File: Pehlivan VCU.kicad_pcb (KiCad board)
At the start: 2 copper layers, 85.7 x 86.6 mm, 58 parts, among them J1 PWR_IN, J2 DEBUG, J3 SD_CARD MODULE, J4 Headlights, J5 Nextion, J6 LORA, J7 Blinker, J8 CAN, J9 Stop, U1 L7805, U2 STM32G431C8Tx, U3 LM1117MP-3.3, U4 BTS432, U5 BTS432, U6 BTS432, U7 BTS432, U8 TJA1051T-3, U9 BTS432, Y1 16MHz 18pF

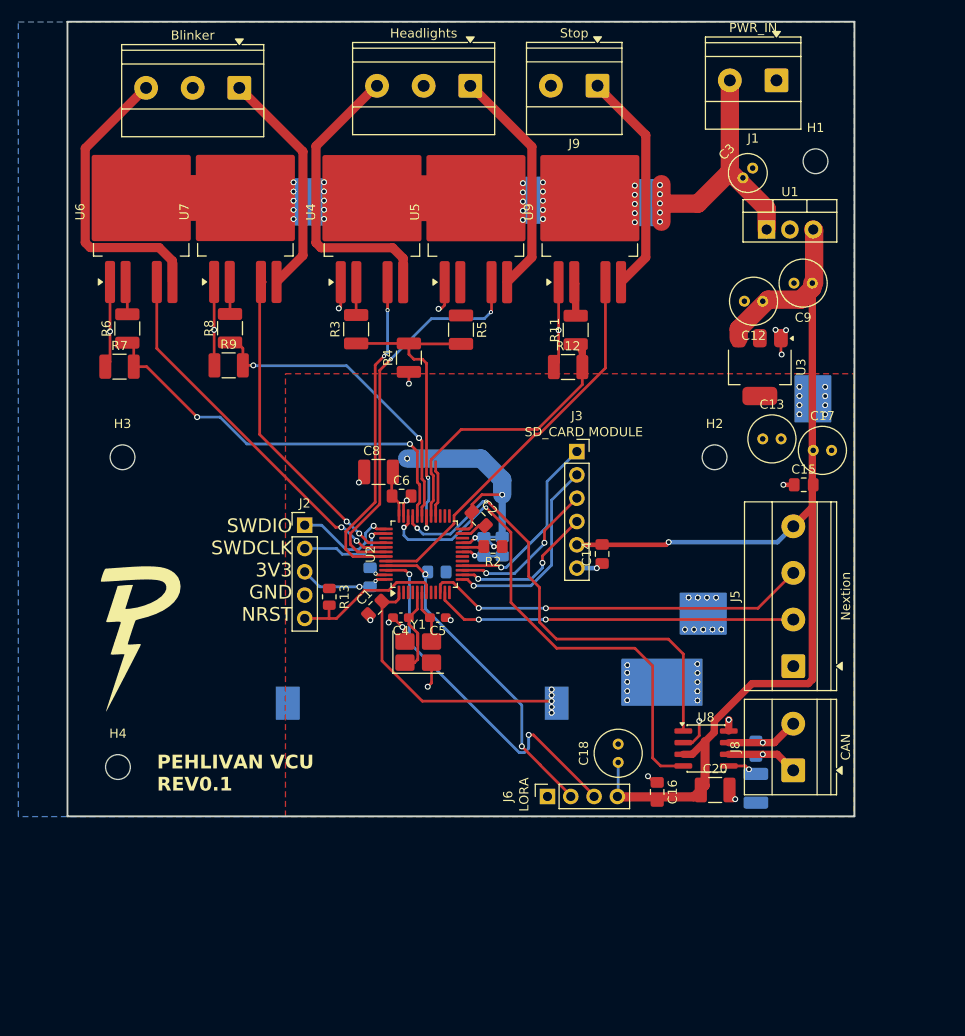
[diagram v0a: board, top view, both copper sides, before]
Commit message: changes
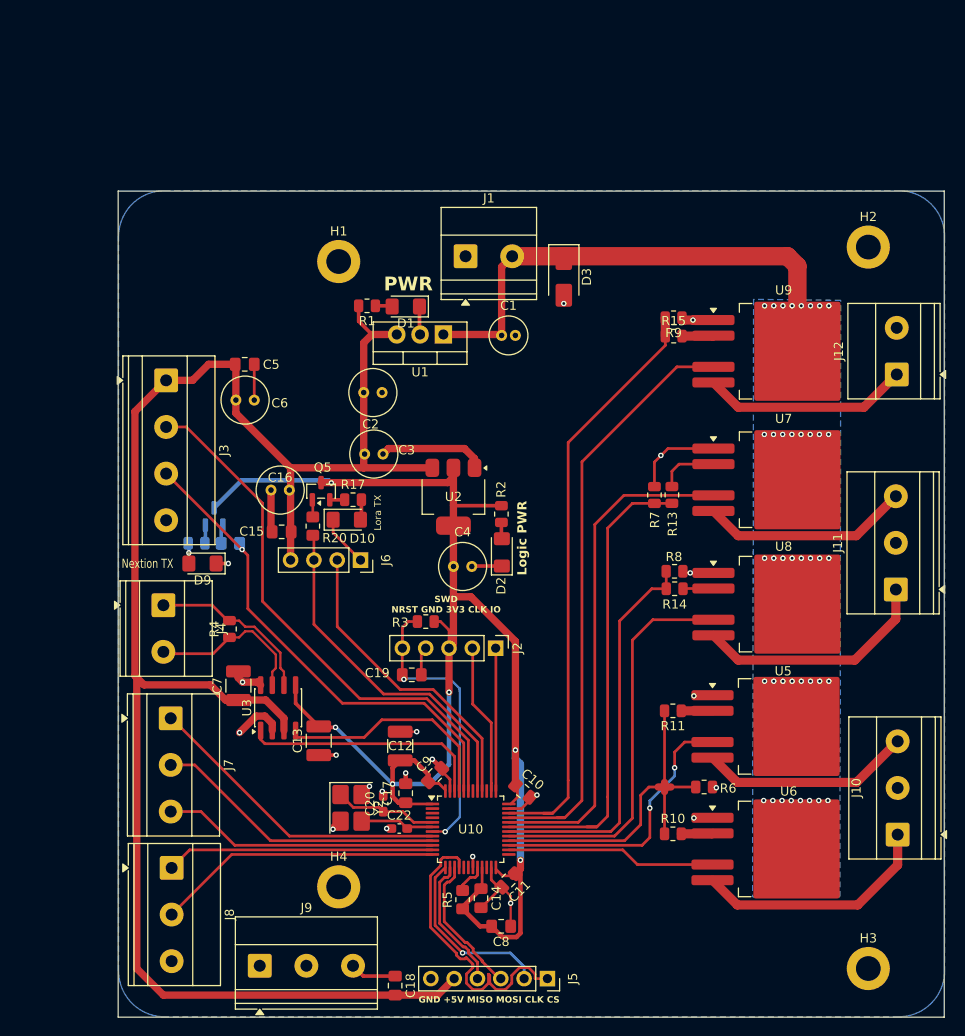
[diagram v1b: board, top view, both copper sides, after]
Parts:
- removed BT1: Battery_Cell, Battery:BatteryHolder_Keystone_1060_1x2032
- removed G***: LOGO, LOGO
- removed R12: 10k, Resistor_SMD:R_1210_3225Metric_Pad1.30x2.65mm_HandSolder
- removed U4: BTS432, Package_TO_SOT_SMD:TO-263-4
- removed Y1: 16MHz 18pF, Crystal:Crystal_SMD_3225-4Pin_3.2x2.5mm_HandSoldering
- added C22: 26pF, Capacitor_SMD:C_0603_1608Metric_Pad1.08x0.95mm_HandSolder, F.Cu at (133.9, 129.4)
- added D1: LED, LED_SMD:LED_1206_3216Metric_Pad1.42x1.75mm_HandSolder, F.Cu at (134.6, 72.6)
- added D10: LED, LED_SMD:LED_1206_3216Metric_Pad1.42x1.75mm_HandSolder, F.Cu at (128.2, 95.8)
- added D2: LED, LED_SMD:LED_1206_3216Metric_Pad1.42x1.75mm_HandSolder, F.Cu at (145.1, 99.4)
- added D3: SMAJ16CA, Diode_SMD:D_SMA, F.Cu at (151.8, 69.3)
- added D9: LED, LED_SMD:LED_1206_3216Metric_Pad1.42x1.75mm_HandSolder, F.Cu at (112.5, 100.6)
- added J10: Headlights, TerminalBlock_Phoenix:TerminalBlock_Phoenix_MKDS-1,5-3-5.08_1x03_P5.08mm_Horizontal, F.Cu at (188.2, 130.1)
- added J11: Blinker, TerminalBlock_Phoenix:TerminalBlock_Phoenix_MKDS-1,5-3-5.08_1x03_P5.08mm_Horizontal, F.Cu at (188.0, 103.4)
- added J12: Stop, TerminalBlock_Phoenix:TerminalBlock_Phoenix_MKDS-1,5-2-5.08_1x02_P5.08mm_Horizontal, F.Cu at (188.1, 80.0)
- added Q4: BC817, Package_TO_SOT_SMD:SOT-23, B.Cu at (113.7, 95.5)
- added Q5: BC817, Package_TO_SOT_SMD:SOT-23, F.Cu at (125.4, 92.7)
- added R14: 4k7, Resistor_SMD:R_0805_2012Metric, F.Cu at (163.9, 103.3)
- added R15: 4k7, Resistor_SMD:R_0805_2012Metric, F.Cu at (163.8, 75.8)
- added R16: 1k, Resistor_SMD:R_0805_2012Metric, B.Cu at (111.8, 98.4)
- added R17: 1k, Resistor_SMD:R_0805_2012Metric, F.Cu at (128.9, 93.6)
- added R19: 4.7K, Resistor_SMD:R_0805_2012Metric_Pad1.20x1.40mm_HandSolder, B.Cu at (115.5, 98.4)
- added R20: 4.7K, Resistor_SMD:R_0805_2012Metric_Pad1.20x1.40mm_HandSolder, F.Cu at (124.5, 96.5)
- added U10: STM32G431C8Tx, Package_QFP:LQFP-48_7x7mm_P0.5mm, F.Cu at (141.7, 129.5)
- added Y2: 16MHz 18pF, Crystal:Crystal_SMD_3225-4Pin_3.2x2.5mm_HandSoldering, F.Cu at (128.7, 127.2)
- C1: value 100nF -> 100uF; footprint Capacitor_SMD:C_0805_2012Metric_Pad1.18x1.45mm_HandSolder -> Capacitor_THT:C_Radial_D4.0mm_H7.0mm_P1.50mm
- C10: moved to F.Cu
- C11: value 10uF -> 100nF; moved to F.Cu
- C12: footprint Capacitor_THT:C_Radial_D5.0mm_H5.0mm_P2.00mm -> Capacitor_SMD:C_1210_3225Metric_Pad1.33x2.70mm_HandSolder
- C13: value 1uF -> 100nF; footprint Capacitor_THT:C_Radial_D5.0mm_H5.0mm_P2.00mm -> Capacitor_SMD:C_1210_3225Metric_Pad1.33x2.70mm_HandSolder
- C16, C2, C6: value 100nF -> 10uF; footprint Capacitor_SMD:C_0805_2012Metric_Pad1.18x1.45mm_HandSolder -> Capacitor_THT:C_Radial_D5.0mm_H5.0mm_P2.00mm
- C17, C18, C9: value 10uF -> 100nF; footprint Capacitor_THT:C_Radial_D5.0mm_H5.0mm_P2.00mm -> Capacitor_SMD:C_0805_2012Metric_Pad1.18x1.45mm_HandSolder
- C19: footprint Capacitor_SMD:C_1210_3225Metric_Pad1.33x2.70mm_HandSolder -> Capacitor_SMD:C_0805_2012Metric_Pad1.18x1.45mm_HandSolder; moved to F.Cu
- C20: value 100nF -> 26pF; footprint Capacitor_SMD:C_1210_3225Metric_Pad1.33x2.70mm_HandSolder -> Capacitor_SMD:C_0603_1608Metric_Pad1.08x0.95mm_HandSolder
- C3: value 100uF -> 10uF; footprint Capacitor_THT:C_Radial_D4.0mm_H7.0mm_P1.50mm -> Capacitor_THT:C_Radial_D5.0mm_H5.0mm_P2.00mm
- C4: value 26pF -> 1uF; footprint Capacitor_SMD:C_0603_1608Metric_Pad1.08x0.95mm_HandSolder -> Capacitor_THT:C_Radial_D5.0mm_H5.0mm_P2.00mm
- C5: value 26pF -> 100nF; footprint Capacitor_SMD:C_0603_1608Metric_Pad1.08x0.95mm_HandSolder -> Capacitor_SMD:C_0805_2012Metric_Pad1.18x1.45mm_HandSolder
- C7: footprint Capacitor_SMD:C_0805_2012Metric_Pad1.18x1.45mm_HandSolder -> Capacitor_SMD:C_1210_3225Metric_Pad1.33x2.70mm_HandSolder; moved to F.Cu
- C8: footprint Capacitor_SMD:C_1210_3225Metric_Pad1.33x2.70mm_HandSolder -> Capacitor_SMD:C_0805_2012Metric_Pad1.18x1.45mm_HandSolder
- H1, H2, H3, H4: footprint MountingHole:MountingHole_2.7mm_M2.5 -> MountingHole:MountingHole_2.7mm_M2.5_DIN965_Pad
- J3: value SD_CARD MODULE -> Nextion; footprint Connector_PinSocket_2.54mm:PinSocket_1x06_P2.54mm_Vertical -> TerminalBlock_Phoenix:TerminalBlock_Phoenix_MKDS-1,5-4-5.08_1x04_P5.08mm_Horizontal
- J4: value Headlights -> CAN; footprint TerminalBlock_Phoenix:TerminalBlock_Phoenix_MKDS-1,5-3-5.08_1x03_P5.08mm_Horizontal -> TerminalBlock_Phoenix:TerminalBlock_Phoenix_MKDS-1,5-2-5.08_1x02_P5.08mm_Horizontal
- J5: value Nextion -> SD_CARD MODULE; footprint TerminalBlock_Phoenix:TerminalBlock_Phoenix_MKDS-1,5-4-5.08_1x04_P5.08mm_Horizontal -> Connector_PinSocket_2.54mm:PinSocket_1x06_P2.54mm_Vertical
- J7: value Blinker -> IN1
- J8: value CAN -> IN2; footprint TerminalBlock_Phoenix:TerminalBlock_Phoenix_MKDS-1,5-2-5.08_1x02_P5.08mm_Horizontal -> TerminalBlock_Phoenix:TerminalBlock_Phoenix_MKDS-1,5-3-5.08_1x03_P5.08mm_Horizontal
- J9: value Stop -> GND; footprint TerminalBlock_Phoenix:TerminalBlock_Phoenix_MKDS-1,5-2-5.08_1x02_P5.08mm_Horizontal -> TerminalBlock_Phoenix:TerminalBlock_Phoenix_MKDS-1,5-3-5.08_1x03_P5.08mm_Horizontal
- R1: value 10k -> 1k; footprint Resistor_SMD:R_0805_2012Metric_Pad1.20x1.40mm_HandSolder -> Resistor_SMD:R_0805_2012Metric; moved to F.Cu
- R10: value 100R -> 4k7; moved to F.Cu
- R11, R7, R9: footprint Resistor_SMD:R_1210_3225Metric_Pad1.30x2.65mm_HandSolder -> Resistor_SMD:R_0805_2012Metric
- R13: value 10k -> 4k7
- R2: value 47R -> 1k; footprint Resistor_SMD:R_0805_2012Metric_Pad1.20x1.40mm_HandSolder -> Resistor_SMD:R_0805_2012Metric
- R3, R6, R8: value 4k7 -> 10k; footprint Resistor_SMD:R_1210_3225Metric_Pad1.30x2.65mm_HandSolder -> Resistor_SMD:R_0805_2012Metric
- R4: value 10k -> 100R; footprint Resistor_SMD:R_1210_3225Metric_Pad1.30x2.65mm_HandSolder -> Resistor_SMD:R_0805_2012Metric
- R5: value 4k7 -> 47R; footprint Resistor_SMD:R_1210_3225Metric_Pad1.30x2.65mm_HandSolder -> Resistor_SMD:R_0805_2012Metric_Pad1.20x1.40mm_HandSolder
- U2: value STM32G431C8Tx -> LM1117MP-3.3; footprint Package_QFP:LQFP-48_7x7mm_P0.5mm -> Package_TO_SOT_SMD:SOT-223-3_TabPin2
- U3: value LM1117MP-3.3 -> TJA1051T-3; footprint Package_TO_SOT_SMD:SOT-223-3_TabPin2 -> Package_SO:SOIC-8_3.9x4.9mm_P1.27mm
- U8: value TJA1051T-3 -> BTS432; footprint Package_SO:SOIC-8_3.9x4.9mm_P1.27mm -> Package_TO_SOT_SMD:TO-263-4
- moved J9 102.7 mm to (118.7, 144.4), turned to 0 degrees
- moved H3 98.5 mm to (185.0, 144.7)
- moved U6 98.5 mm to (175.7, 131.7), turned to 0 degrees
- moved R6 80.3 mm to (167.1, 124.9), turned to 180 degrees
- moved J7 69.1 mm to (109.0, 117.4), turned to -90 degrees
- moved J8 68.5 mm to (109.1, 133.7), turned to -90 degrees
- moved C9 67.5 mm to (137.8, 123.6), turned to 45 degrees
- moved J4 65.7 mm to (108.2, 105.1), turned to -90 degrees
- moved U7 65.5 mm to (175.8, 91.5), turned to 0 degrees
- moved U5 65.3 mm to (175.7, 118.3), turned to 0 degrees
- moved U3 64.3 mm to (120.7, 116.3), turned to 90 degrees
- moved C12 62.5 mm to (134.0, 120.5), turned to -90 degrees
- moved R5 62.1 mm to (140.8, 137.2), turned to 90 degrees
- moved R7 59.9 mm to (161.7, 93.1), turned to -90 degrees
- moved C13 58.5 mm to (125.1, 119.9), turned to 90 degrees
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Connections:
- C1 pad 1: GND -> VCC
- C1 pad 2: /VBAT -> GND
- C11 pad 1: GND -> +3V3
- C11 pad 2: +3V3 -> GND
- C12 pad 1: +5V -> GND
- C12 pad 2: GND -> +3V3
- C13 pad 1: +3V3 -> GND
- C13 pad 2: GND -> +3V3
- C14 pad 1: GND -> +3V3
- C14 pad 2: +5V -> GND
- C16 pad 1: GND -> +5V
- C16 pad 2: +5V -> GND
- C17 pad 1: +5V -> +3V3
- C18 pad 1: +5V -> GND
- C18 pad 2: GND -> +5V
- C19 pad 1: GND -> /NRST
- C19 pad 2: +3V3 -> GND
- C2 pad 1: +3V3 -> +5V
- C20 pad 1: +5V -> /HSE_IN
- C3 pad 1: VCC -> +5V
- C4 pad 1: /HSE_IN -> +3V3
- C5 pad 2: /HSE_OUT -> +5V
- C6 pad 1: +3V3 -> +5V
- C7 pad 1: +3V3 -> +5V
- C9 pad 1: +5V -> +3V3
- J3 pad 1: /SPI_CS -> +5V
- J3 pad 2: /SPICK -> /UART1_RX
- J3 pad 3: /SPIMOSI -> /UART1_TX
- J3 pad 4: /SPIMISO -> GND
- J4 pad 1: /R_HL_OUT -> /CANN
- J4 pad 2: GND -> /CANP
- J5 pad 1: GND -> /SPI_CS
- J5 pad 2: /UART2_RX -> /SPICK
- J5 pad 3: /UART2_TX -> /SPIMOSI
- J5 pad 4: +5V -> /SPIMISO
- J6 pad 2: /UART3_RX -> /UART2_RX
- J6 pad 3: /UART3_TX -> /UART2_TX
- J7 pad 1: /R_BL_OUT -> /Left_Signal_IN
- J7 pad 2: GND -> /Right_Signal_IN
- J7 pad 3: /L_BL_OUT -> /Hazards_IN
- J8 pad 1: Net-(J8-Pin_1) -> /Headlights_IN
- J8 pad 2: Net-(J8-Pin_2) -> /Brake_IN
- J9 pad 1: /STOP_OUT -> GND
- R1 pad 1: GND -> Net-(D1-A)
- R1 pad 2: /UART3_RX -> +5V
- R10 pad 1: Net-(J8-Pin_2) -> /F_Headlights
- R10 pad 2: Net-(J8-Pin_1) -> Net-(U6-IN)
- R11 pad 1: /F_BrakeLights -> Net-(U5-IN)
- R11 pad 2: Net-(U9-IN) -> /F_Headlights
- R13 pad 1: +3V3 -> /L_Blinker
- R13 pad 2: /NRST -> Net-(U7-IN)
- R2 pad 1: +3V3 -> Net-(D2-A)
- R2 pad 2: /VREF -> +3V3
- R3 pad 1: /F_Headlights -> +3V3
- R3 pad 2: Net-(U4-IN) -> /NRST
- R4 pad 1: GND -> /CANP
- R4 pad 2: /F_Headlights -> /CANN
- R5 pad 1: Net-(U5-IN) -> +3V3
- R5 pad 2: /F_Headlights -> /VREF
- R6 pad 1: /L_Blinker -> GND
- R6 pad 2: Net-(U6-IN) -> /F_Headlights
- R8 pad 1: /R_Blinker -> GND
- R8 pad 2: Net-(U7-IN) -> /R_Blinker
- R9 pad 2: /R_Blinker -> /F_BrakeLights
- U2 pad 1: /VBAT -> GND
- U2 pad 2: unconnected-(U2-PC13-Pad2) -> +3V3
- U2 pad 3: unconnected-(U2-PC14-Pad3) -> +5V
- U3 pad 1: GND -> /FDCAN_RX
- U3 pad 2: +3V3 -> GND
- U6 pad 4: /L_BL_FAULT -> /L_HL_FAULT
- U6 pad 5: /L_BL_OUT -> /L_HL_OUT
- U7 pad 4: /R_BL_FAULT -> /L_BL_FAULT
- U7 pad 5: /R_BL_OUT -> /L_BL_OUT
- U8 pad 1: /FDCAN_RX -> GND
- U8 pad 2: GND -> Net-(U8-IN)
- U8 pad 3: +5V -> VCC
- U8 pad 4: /FDCAN_TX -> /R_BL_FAULT
- U8 pad 5: +3V3 -> /R_BL_OUT
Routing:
- net +3V3: track 49.3 -> 174.7 mm, vias 34 -> 6
- net +5V: track 124.5 -> 190.2 mm, vias 1 -> 0
- net /UART1_RX: track 0.00 -> 59.4 mm
- net /UART1_TX: track 0.00 -> 53.2 mm, vias 0 -> 1
- net /UART3_TX: track 39.9 -> 0.00 mm, vias 2 -> 0
- net /UART3_RX: track 35.6 -> 0.00 mm, vias 2 -> 0
- net /F_BrakeLights: track 30.9 -> 64.9 mm
- net /Left_Signal_IN: track 0.00 -> 33.7 mm
- net /VBAT: track 32.7 -> 0.00 mm, vias 5 -> 0
- net /Right_Signal_IN: track 0.00 -> 31.8 mm
- net /Brake_IN: track 0.00 -> 31.1 mm
- net /FDCAN_TX: track 56.4 -> 25.4 mm, vias 2 -> 0
- net /Hazards_IN: track 0.00 -> 29.9 mm
- net /Headlights_IN: track 0.00 -> 29.2 mm
- net GND: track 64.0 -> 92.1 mm, vias 24 -> 21
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- added copper zone on B.Cu, net VCC
- removed copper zone on F.Cu, net +3V3
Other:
- board size 85.7 x 86.6 mm -> 90 x 90 mm
- board text added: "5V"
- board text added: "Brake IN"
- board text added: "CAN"
- board text added: "GND"
- board text added: "GND +5V MISO MOSI CLK CS"
- board text added: "H"
- board text added: "Hazards In"
- board text added: "Headlights"
- board text added: "L"
- board text added: "Left Blinker"
- board text added: "Left Headlight"
- board text added: "Left Signal In"
- board text added: "Logic PWR"
- board text added: "Lora TX"
- board text added: "Nextion Output"
- board text added: "Nextion TX"
- board text added: "PWR"
- board text added: "RX"
- board text added: "Right Blinker"
- board text added: "Right Headlight"
- board text added: "Right Signal In"
- board text added: "SWD NRST GND 3V3 CLK IO"
- board text added: "Stop"
- board text added: "TX"
- board text removed: "Designer: Yener S. Güneş Electronics Team: person name surname 1 person name surname 1 person name surname 1 Electrical Team person name surname 1 person name surname 1 person name surname 1 Software Team person name surname 1 person name surname 1 person name surname 1"
- board text removed: "PEHLIVAN VCU REV0.1"
- board text removed: "SWDIO SWDCLK 3V3 GND NRST"
